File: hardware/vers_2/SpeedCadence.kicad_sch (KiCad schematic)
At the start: 39 parts, among them J1 Conn_ST_STDC14, J2 USB_C_Receptacle_USB2.0_16P, J3 Conn_01x03_Pin, J4 Conn_01x02_Pin, J5 Conn_01x04_Pin, J6 Conn_01x02_Pin, SW2 SW_Push, SW3 SW_Push, U2 STM32F103C8Tx, U3 TCAN3414DR, U4 TPSM861253RDXR, Y1 CSTNE8M00G52Z000R0

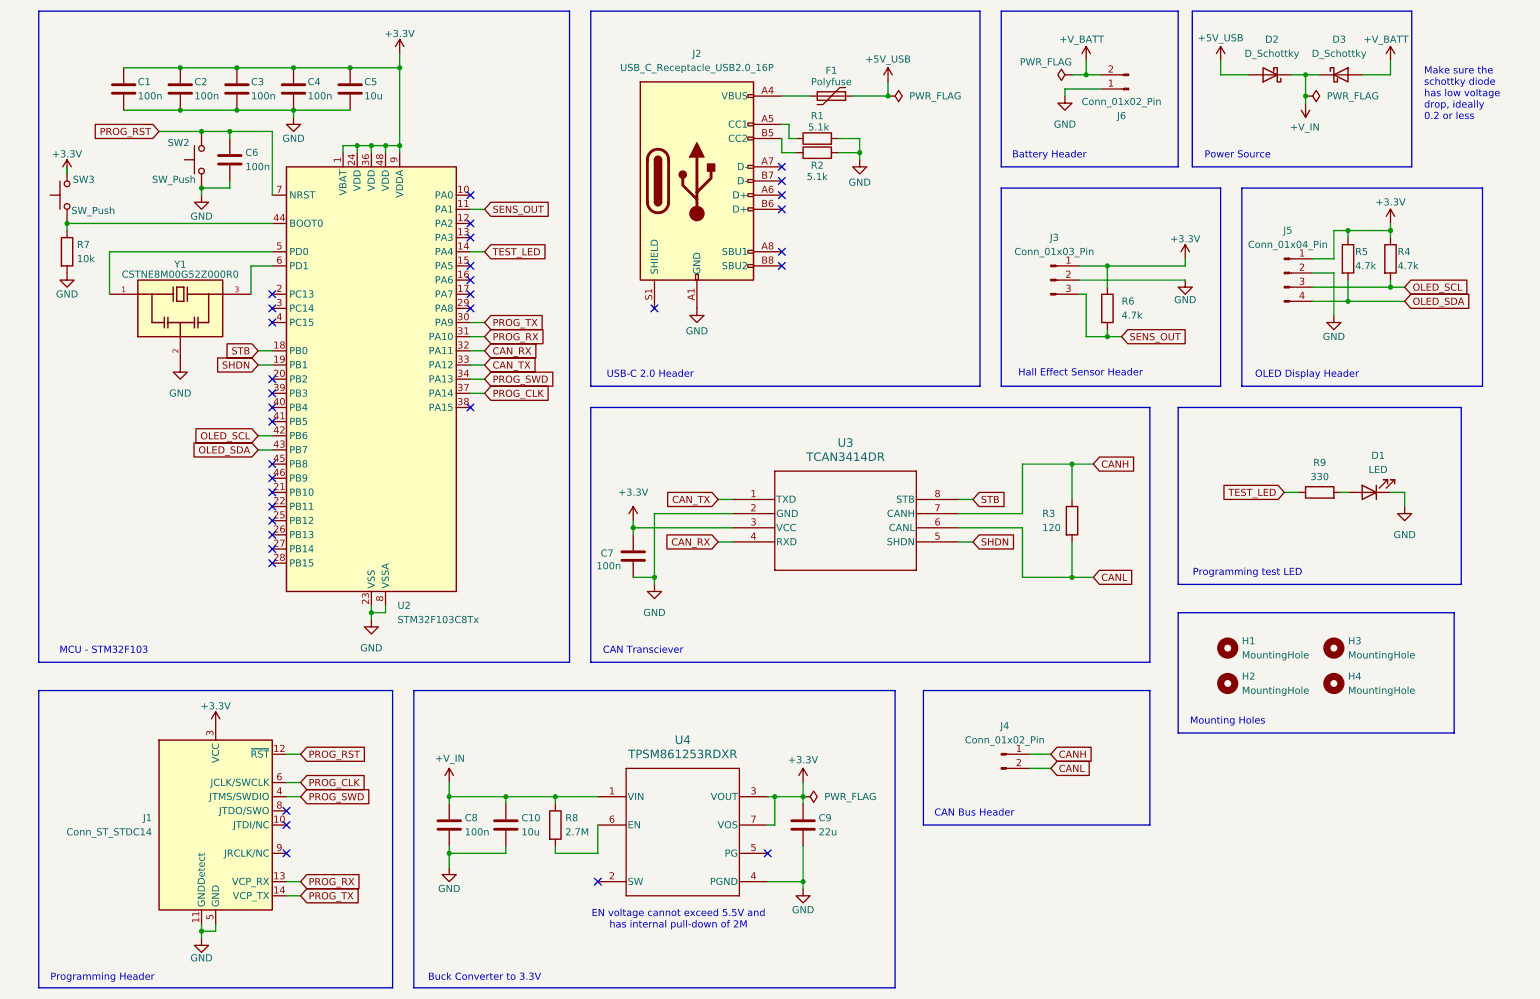
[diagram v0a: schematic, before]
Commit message: Added manufacturers and manufacturer part numbers
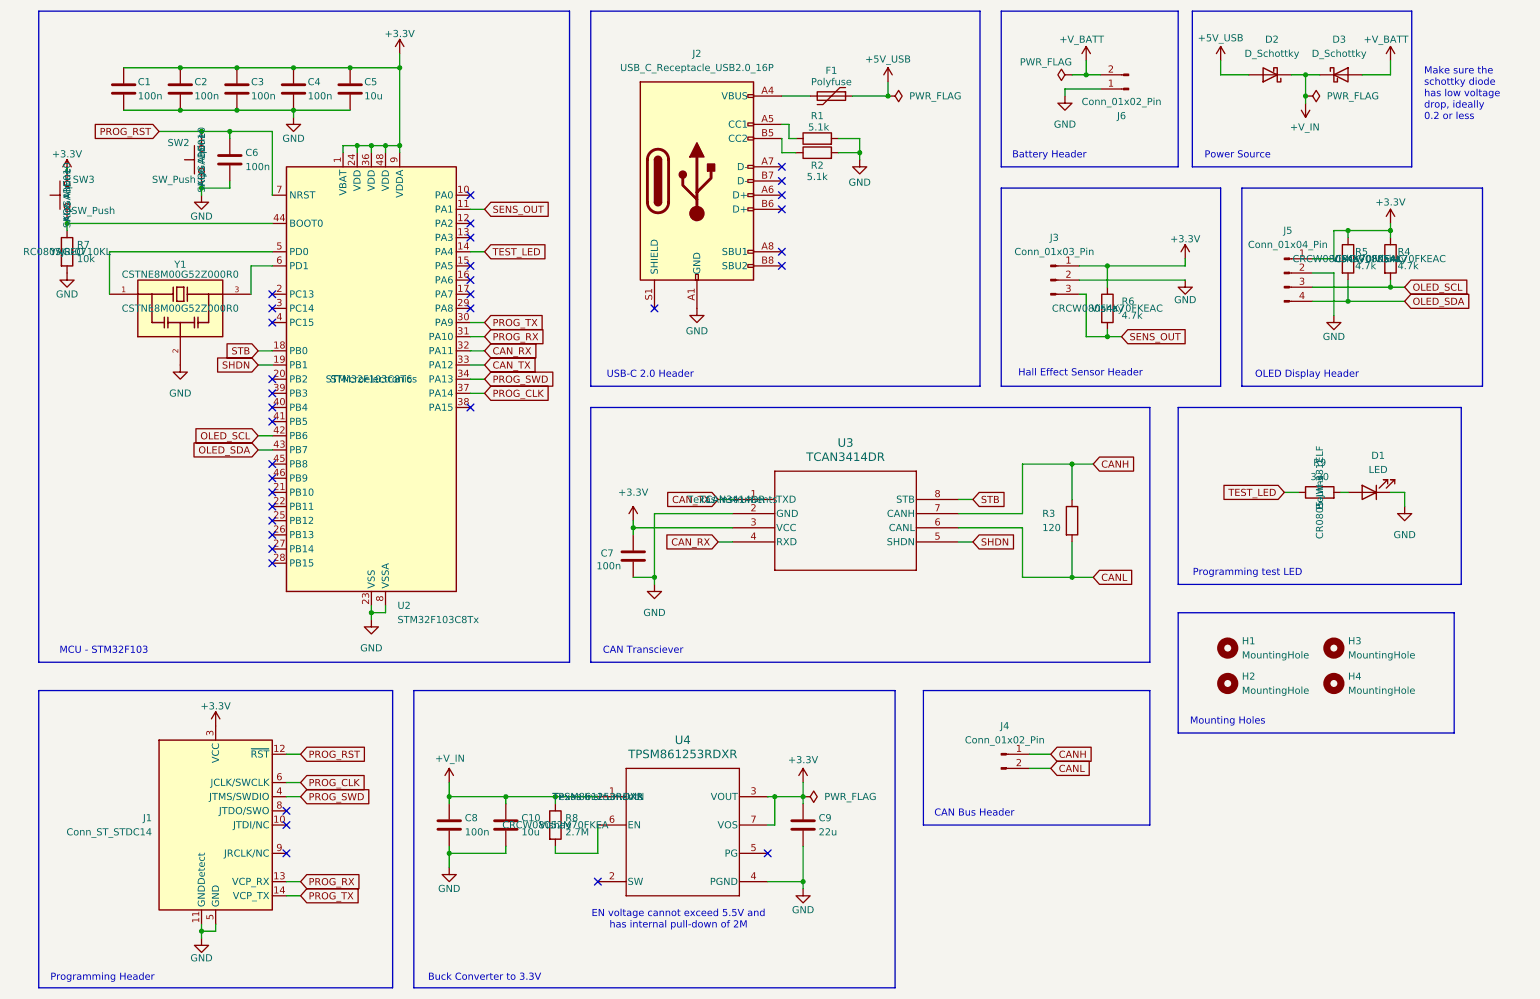
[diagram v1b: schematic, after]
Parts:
- C1, C2, C3, C4, C6, C7, C8: Manufacturer Part Number CC0805KRX7R9BB104 -> CC0805KRX7R9BB104
- C9: Manufacturer Part Number GRM21BZ71A226ME15L -> GRM21BZ71A226ME15L
- D1: Manufacturer Part Number 5975906507F -> 5975906507F
- J1: Manufacturer Part Number FTSH-107-01-L-DV-K-A -> FTSH-107-01-L-DV-K-A
- J2: Manufacturer Part Number DX07S016JA3R1500 -> DX07S016JA3R1500
- J4, J6: Manufacturer Part Number B2B-XH-A-BK(LF)(SN) -> B2B-XH-A-BK(LF)(SN)
- J5: Manufacturer Part Number B4B-XH-A(LF)(SN) -> B4B-XH-A(LF)(SN)
- R3: MANUFACTURER Vishay / Sfernice -> Susumu; Manufacturer Part Number P0603Y60R0BBT -> RG2012N-121-W-T1
- R4, R5, R6: MANUFACTURER (none) -> Vishay; Manufacturer Part Number (none) -> CRCW08054K70FKEAC
- R7: MANUFACTURER (none) -> YAGEO; Manufacturer Part Number (none) -> RC0805JR-0710KL
- R8: MANUFACTURER (none) -> Vishay; Manufacturer Part Number (none) -> CRCW08052M70FKEA
- R9: MANUFACTURER (none) -> Bourns; Manufacturer Part Number (none) -> CR0805-JW-331ELF
- SW2, SW3: MANUFACTURER (none) -> Alps Alpine; Manufacturer Part Number (none) -> SKQGABE010
- U2: MANUFACTURER (none) -> STMicroelectronics; Manufacturer Part Number (none) -> STM32F103C8T6
- U3: MANUFACTURER (none) -> Texas Instruments; Manufacturer Part Number (none) -> TCAN3414DR
- U4: MANUFACTURER (none) -> Texas Instruments; Manufacturer Part Number (none) -> TPSM861253RDXR
- Y1: MANUFACTURER Murata -> Murata Electronics; Manufacturer Part Number (none) -> CSTNE8M00G52Z000R0
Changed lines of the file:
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@@
 			)
 		)
-		(property "Manufacturer Part Number" " B2B-XH-A-BK(LF)(SN)"
+		(property "Manufacturer Part Number" "B2B-XH-A-BK(LF)(SN)"
 			(at 213.36 30.48 0)
 			(effects
@@
 			)
 		)
-		(property "Manufacturer Part Number" ""
+		(property "Manufacturer Part Number" "CRCW08054K70FKEAC"
+			(at 252.73 60.96 0)
+			(effects
+				(font
+					(size 1.27 1.27)
+				)
+			)
+		)
+		(property "MANUFACTURER" "Vishay"
 			(at 252.73 60.96 0)
 			(effects
@@
 			)
 		)
-		(property "Manufacturer Part Number" ""
+		(property "Manufacturer Part Number" "CRCW08052M70FKEA"
+			(at 110.49 162.56 0)
+			(effects
+				(font
+					(size 1.27 1.27)
+				)
+			)
+		)
+		(property "MANUFACTURER" "Vishay"
 			(at 110.49 162.56 0)
 			(effects
@@
 			)
 		)
-		(property "Manufacturer Part Number" " CC0805KRX7R9BB104"
+		(property "Manufacturer Part Number" "CC0805KRX7R9BB104"
 			(at 91.44 162.56 0)
 			(effects
@@
 			)
 		)
-		(property "Manufacturer Part Number" ""
+		(property "Manufacturer Part Number" "STM32F103C8T6"
+			(at 77.47 82.55 0)
+			(effects
+				(font
+					(size 1.27 1.27)
+				)
+			)
+		)
+		(property "MANUFACTURER" "STMicroelectronics"
 			(at 77.47 82.55 0)
 			(effects
@@
 			)
 		)
-		(property "Manufacturer Part Number" " CC0805KRX7R9BB104"
+		(property "Manufacturer Part Number" "CC0805KRX7R9BB104"
 			(at 52.07 43.18 0)
 			(effects
@@
 			)
 		)
-		(property "Manufacturer Part Number" " CC0805KRX7R9BB104"
+		(property "Manufacturer Part Number" "CC0805KRX7R9BB104"
 			(at 63.5 30.48 0)
 			(effects
@@
 			)
 		)
-		(property "Manufacturer Part Number" ""
+		(property "Manufacturer Part Number" "TPSM861253RDXR"
+			(at 118.11 157.48 0)
+			(effects
+				(font
+					(size 1.27 1.27)
+				)
+			)
+		)
+		(property "MANUFACTURER" "Texas Instruments"
 			(at 118.11 157.48 0)
 			(effects
@@
 			)
 		)
-		(property "Manufacturer Part Number" ""
+		(property "Manufacturer Part Number" "CRCW08054K70FKEAC"
+			(at 209.55 69.85 0)
+			(effects
+				(font
+					(size 1.27 1.27)
+				)
+			)
+		)
+		(property "MANUFACTURER" "Vishay"
 			(at 209.55 69.85 0)
 			(effects
@@
 			)
 		)
-		(property "Manufacturer Part Number" " CC0805KRX7R9BB104"
+		(property "Manufacturer Part Number" "CC0805KRX7R9BB104"
 			(at 43.18 30.48 0)
 			(effects
@@
 			)
 		)
-		(property "Manufacturer Part Number" " FTSH-107-01-L-DV-K-A"
+		(property "Manufacturer Part Number" "FTSH-107-01-L-DV-K-A"
 			(at 49.53 162.56 0)
 			(effects
@@
 			)
 		)
-		(property "MANUFACTURER" "Murata"
+		(property "MANUFACTURER" "Murata Electronics"
 			(at 43.18 69.85 0)
 			(effects
@@
 			)
 		)
-		(property "Manufacturer Part Number" ""
+		(property "Manufacturer Part Number" "CSTNE8M00G52Z000R0"
 			(at 43.18 69.85 0)
 			(effects
@@
 			)
 		)
-		(property "Manufacturer Part Number" " 5975906507F"
+		(property "Manufacturer Part Number" "5975906507F"
 			(at 256.54 102.87 0)
 			(effects
@@
 			)
 		)
-		(property "Manufacturer Part Number" ""
+		(property "Manufacturer Part Number" "SKQGABE010"
+			(at 22.86 49.53 0)
+			(effects
+				(font
+					(size 1.27 1.27)
+				)
+			)
+		)
+		(property "MANUFACTURER" "Alps Alpine"
 			(at 22.86 49.53 0)
 			(effects
@@
 			)
 		)
-		(property "Manufacturer Part Number" " CC0805KRX7R9BB104"
+		(property "Manufacturer Part Number" "CC0805KRX7R9BB104"
 			(at 124.46 114.3 0)
 			(effects
@@
 			)
 		)
-		(property "Manufacturer Part Number" " B4B-XH-A(LF)(SN)"
+		(property "Manufacturer Part Number" "B4B-XH-A(LF)(SN)"
 			(at 241.3 63.5 0)
 			(effects
@@
 			)
 		)
-		(property "Manufacturer Part Number" ""
+		(property "Manufacturer Part Number" "TCAN3414DR"
+			(at 142.24 104.14 0)
+			(effects
+				(font
+					(size 1.27 1.27)
+				)
+			)
+		)
+		(property "MANUFACTURER" "Texas Instruments"
 			(at 142.24 104.14 0)
 			(effects
@@
 			)
 		)
-		(property "Manufacturer Part Number" ""
+		(property "Manufacturer Part Number" "CR0805-JW-331ELF"
+			(at 247.65 102.87 0)
+			(effects
+				(font
+					(size 1.27 1.27)
+				)
+			)
+		)
+		(property "MANUFACTURER" "Bourns"
 			(at 247.65 102.87 0)
 			(effects
@@
 			)
 		)
-		(property "Manufacturer Part Number" " GRM21BZ71A226ME15L"
+		(property "Manufacturer Part Number" "GRM21BZ71A226ME15L"
 			(at 154.94 162.56 0)
 			(effects
@@
 			)
 		)
-		(property "Manufacturer Part Number" " B2B-XH-A-BK(LF)(SN)"
+		(property "Manufacturer Part Number" "B2B-XH-A-BK(LF)(SN)"
 			(at 190.5 149.86 0)
 			(effects
@@
 			)
 		)
-		(property "Manufacturer Part Number" " CC0805KRX7R9BB104"
+		(property "Manufacturer Part Number" "CC0805KRX7R9BB104"
 			(at 53.34 30.48 0)
 			(effects
@@
 			)
 		)
-		(property "Manufacturer Part Number" " CC0805KRX7R9BB104"
+		(property "Manufacturer Part Number" "CC0805KRX7R9BB104"
 			(at 33.02 30.48 0)
 			(effects
@@
 			)
 		)
-		(property "Manufacturer Part Number" ""
+		(property "Manufacturer Part Number" "SKQGABE010"
+			(at 46.99 43.18 0)
+			(effects
+				(font
+					(size 1.27 1.27)
+				)
+			)
+		)
+		(property "MANUFACTURER" "Alps Alpine"
 			(at 46.99 43.18 0)
 			(effects
@@
 			)
 		)
-		(property "Manufacturer Part Number" " DX07S016JA3R1500"
+		(property "Manufacturer Part Number" "DX07S016JA3R1500"
 			(at 135.89 46.99 0)
 			(effects
@@
 			)
 		)
-		(property "Manufacturer Part Number" ""
+		(property "Manufacturer Part Number" "RC0805JR-0710KL"
+			(at 22.86 59.69 0)
+			(effects
+				(font
+					(size 1.27 1.27)
+				)
+			)
+		)
+		(property "MANUFACTURER" "YAGEO"
 			(at 22.86 59.69 0)
 			(effects
@@
 			)
 		)
-		(property "Manufacturer Part Number" "P0603Y60R0BBT"
+		(property "Manufacturer Part Number" "RG2012N-121-W-T1"
 			(at 203.2 107.95 0)
 			(effects
@@
 			)
 		)
-		(property "MANUFACTURER" "Vishay / Sfernice"
+		(property "MANUFACTURER" "Susumu"
 			(at 203.2 107.95 0)
 			(effects
@@
 			)
 		)
-		(property "Manufacturer Part Number" ""
+		(property "Manufacturer Part Number" "CRCW08054K70FKEAC"
+			(at 260.35 60.96 0)
+			(effects
+				(font
+					(size 1.27 1.27)
+				)
+			)
+		)
+		(property "MANUFACTURER" "Vishay"
 			(at 260.35 60.96 0)
 			(effects
